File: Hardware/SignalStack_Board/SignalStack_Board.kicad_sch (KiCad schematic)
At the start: 68 parts, among them J1 Molex_uF_SV_06, J2 RJ45_LED_Shielded, J3 Molex_uF_SV_06, Q1 SI4156DY, Q2 SI4156DY, Q3 SI4156DY, Q4 SI4156DY, Q5 SI4156DY, Q6 SI4156DY, Q7 SI4156DY, Q8 SI4156DY, U1 OKI, U2 SMAJ12CA, U3 Teensy4.1_DEV-16771, U4 TSR_1-2450, U5 IRS2005S, U6 IRS2005S, U7 MMC5633NJL, U8 IRS2005S, U9 IRS2005S

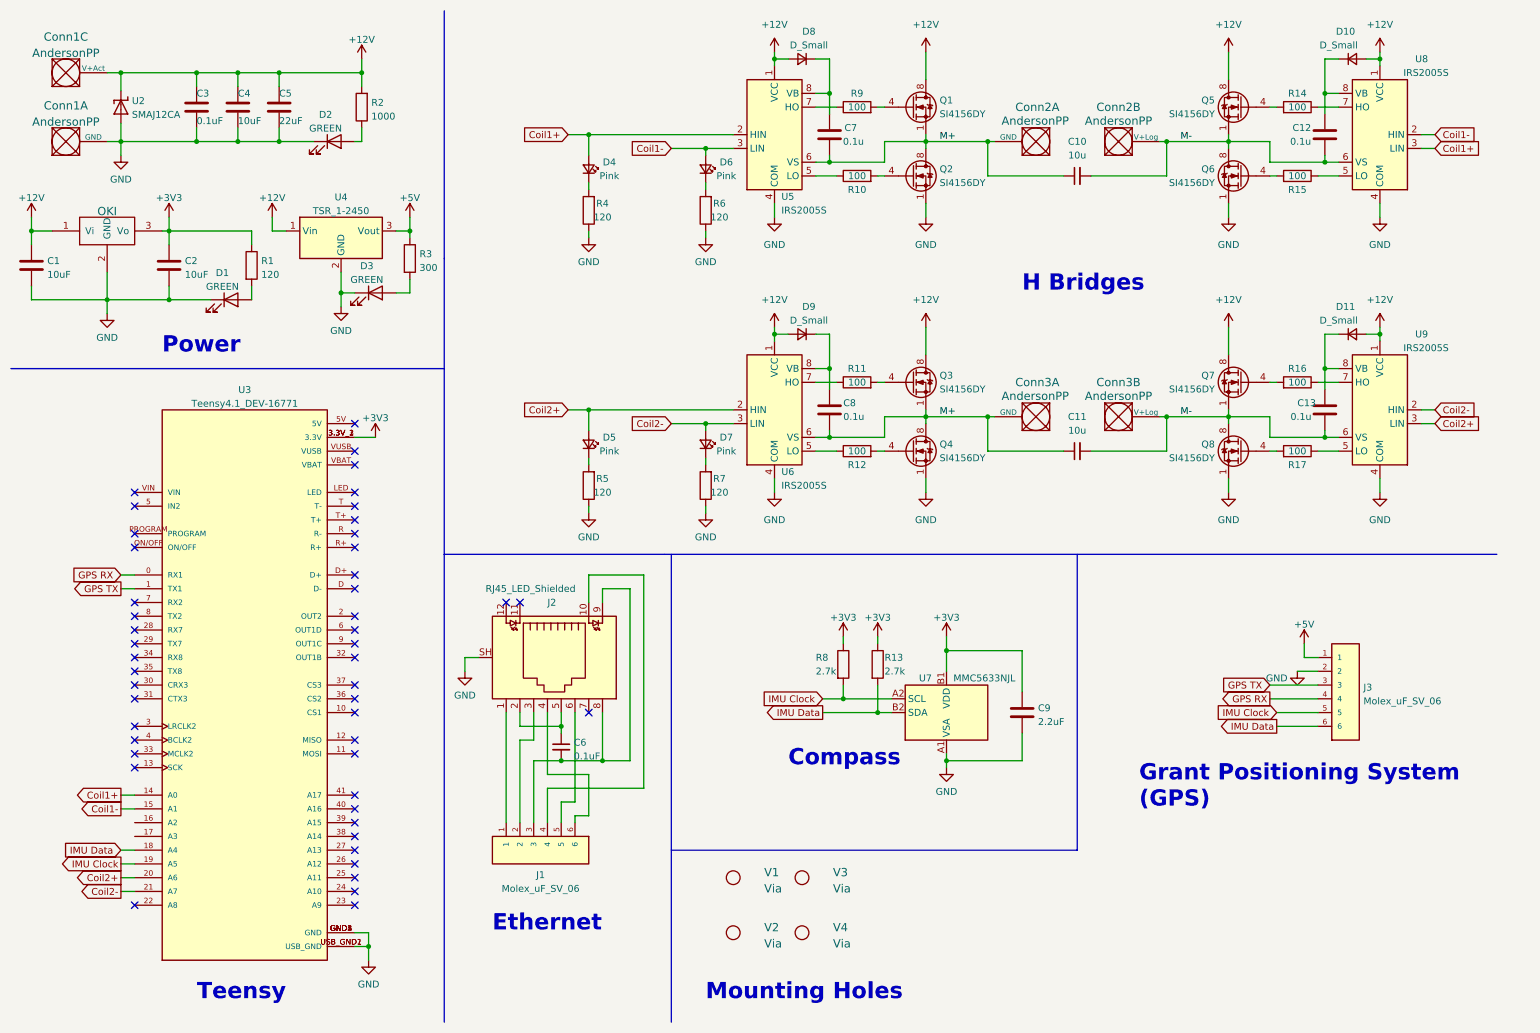
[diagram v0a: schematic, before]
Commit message: Finished schematic
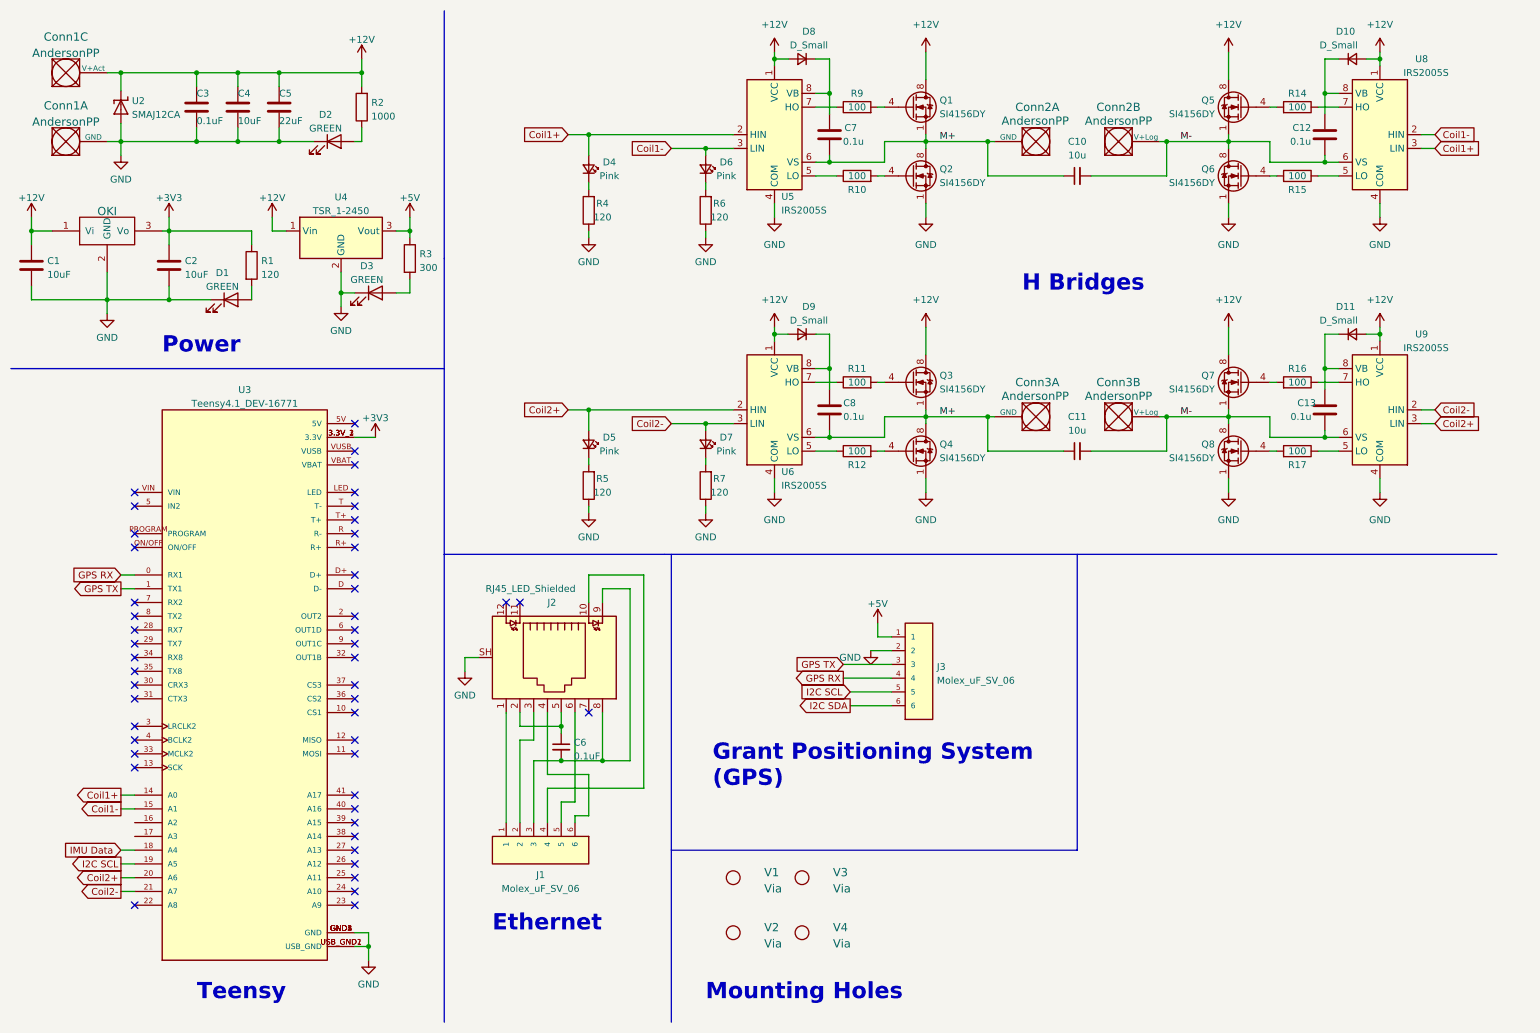
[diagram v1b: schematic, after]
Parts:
- removed C9: 2.2uF, Capacitor_SMD:C_0603_1608Metric_Pad1.08x0.95mm_HandSolder, symbol Device:C
- removed R13, R8: 2.7k, Resistor_SMD:R_0603_1608Metric_Pad0.98x0.95mm_HandSolder, symbol Device:R
- removed U7: MMC5633NJL, Package_BGA:WLP-4_0.86x0.86mm_P0.4mm, symbol Sensor_Magnetic:MMC5633NJL
- U4: footprint Converter_DCDC:Converter_DCDC_TRACO_TSR-1_THT -> MRDT_Devices:TSR_1-2433
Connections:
- net IMU Data: no longer J3.6
- net IMU Clock renamed I2C SCL
- new net I2C SDA: J3.6
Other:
- note removed: "Compass"
- moved on the sheet: J3
